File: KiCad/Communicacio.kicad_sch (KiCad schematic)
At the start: 0 parts

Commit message: Procesament i comunicació
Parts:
- added C7: 100nF, symbol Device:C
- added J2: USB_B_Micro, symbol Connector:USB_B_Micro
- added R11: 10K, symbol Device:R
- added U5: FT232RL, Package_SO:SSOP-28_5.3x10.2mm_P0.65mm, symbol Interface_USB:FT232RL
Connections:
- new net: J2.2 (D-), U5.16 (USBD-)
- new net: J2.3 (D+), U5.15 (USBD+)
- new net: C7.2, U5.17 (3V3OUT)
- new net: R11.2, U5.19 (~{RESET})
- new net GND: C7.1, J2.5 (GND), J2.6 (Shield), U5.18 (GND), U5.21 (GND), U5.25 (AGND), U5.26 (TEST), U5.7 (GND)
- new net GPIO: U5.10 (DCD), U5.11 (CTS), U5.2 (DTR), U5.3 (RTS), U5.6 (RI), U5.9 (DCR)
- new net U1RX: U5.1 (TXD)
- new net U1TX: U5.5 (RXD)
- new net VCC: J2.1 (VBUS), R11.1, U5.20 (VCC), U5.4 (VCCIO)
- no-connect marks 0 -> 8
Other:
- note added: "USART"

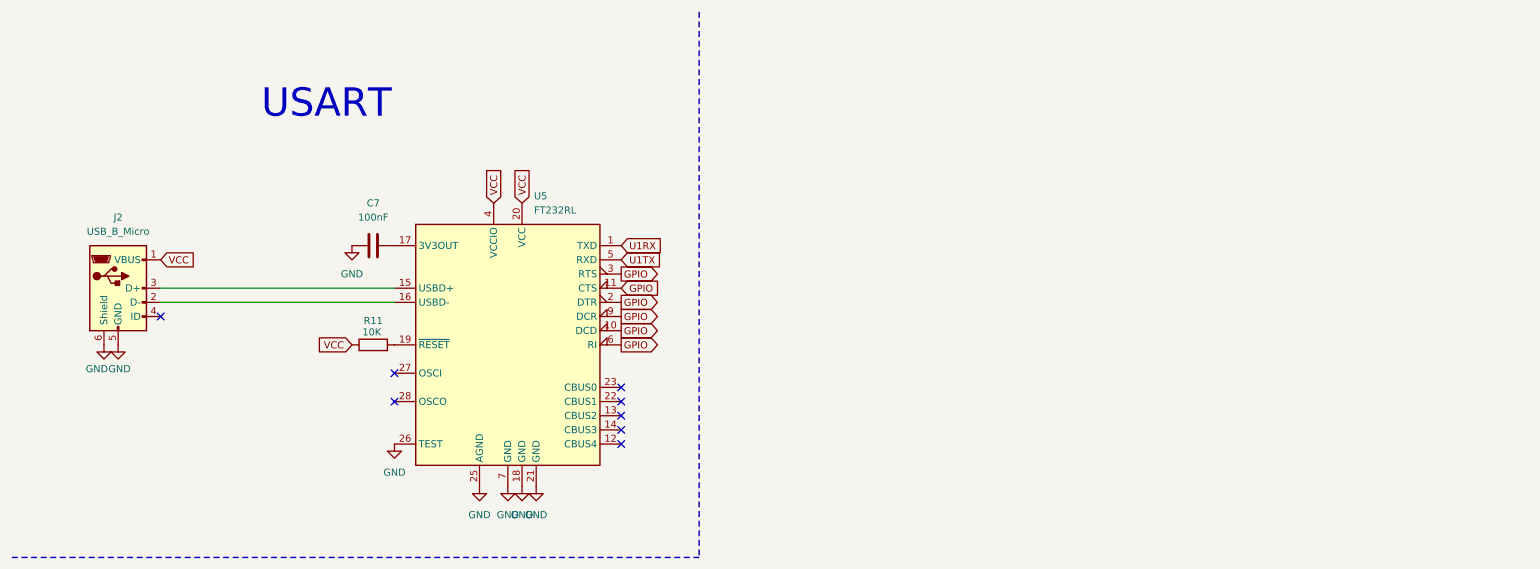
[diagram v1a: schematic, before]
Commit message: botonera, datashet usart
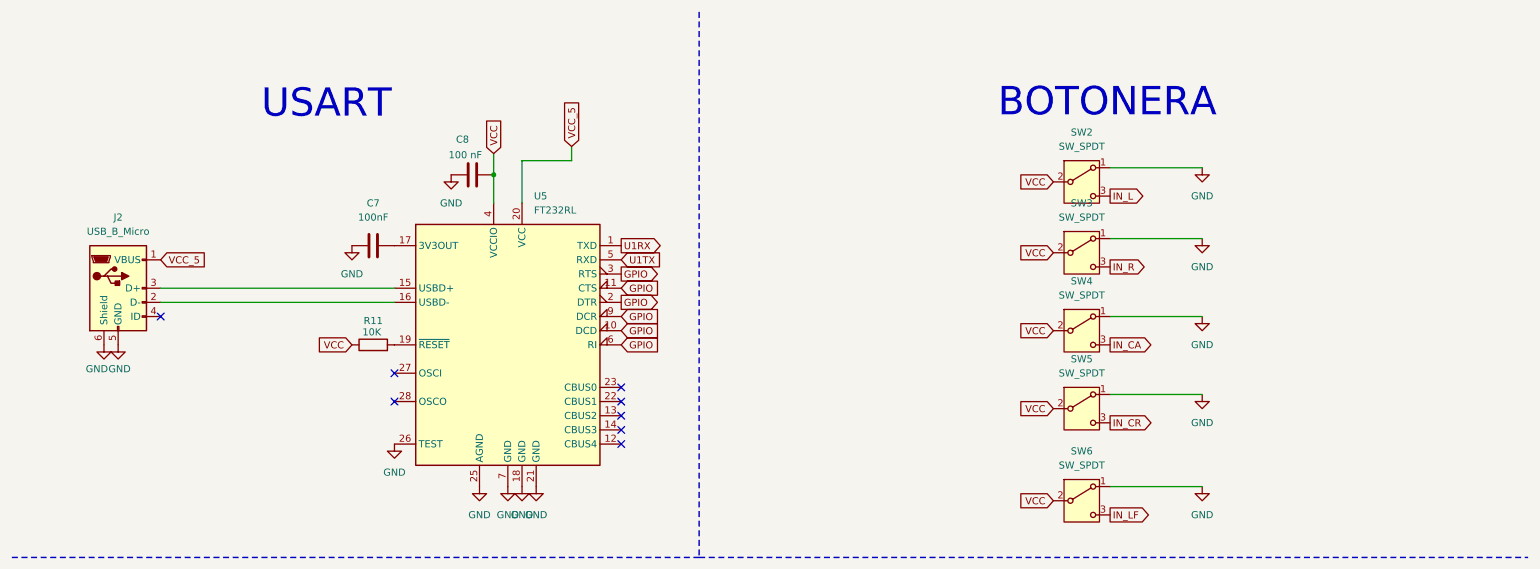
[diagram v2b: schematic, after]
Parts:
- added C8: 100 nF, symbol Device:C
- added SW2, SW3, SW4, SW5, SW6: SW_SPDT, symbol Switch:SW_SPDT
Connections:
- net GND: now also C8.1, SW2.1 (A), SW3.1 (A), SW4.1 (A), SW5.1 (A), SW6.1 (A)
- net VCC: now also C8.2, SW2.2 (B), SW3.2 (B), SW4.2 (B), SW5.2 (B), SW6.2 (B); no longer J2.1 (VBUS), U5.20 (VCC)
- new net IN_CA: SW4.3 (C)
- new net IN_CR: SW5.3 (C)
- new net IN_L: SW2.3 (C)
- new net IN_LF: SW6.3 (C)
- new net IN_R: SW3.3 (C)
- new net VCC_5: J2.1 (VBUS), U5.20 (VCC)
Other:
- note added: "BOTONERA"
